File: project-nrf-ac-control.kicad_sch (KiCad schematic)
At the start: 8 parts, among them J1 SM04B-SRSS-TB(LF)(SN), Q1 SI2312BDS-T1-E3, U1 Pink Panda

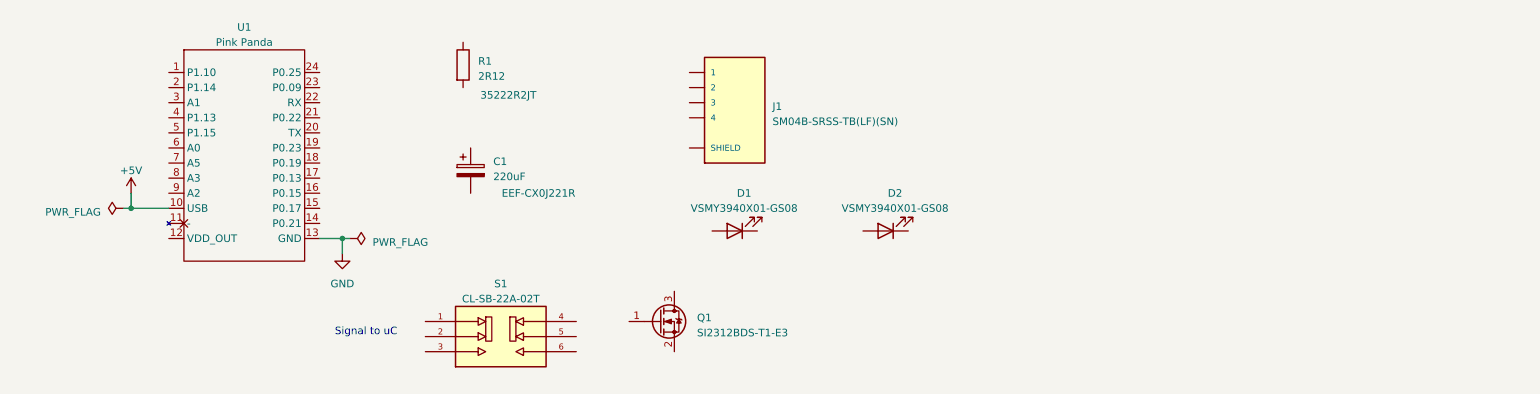
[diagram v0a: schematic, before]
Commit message: First draft schematic
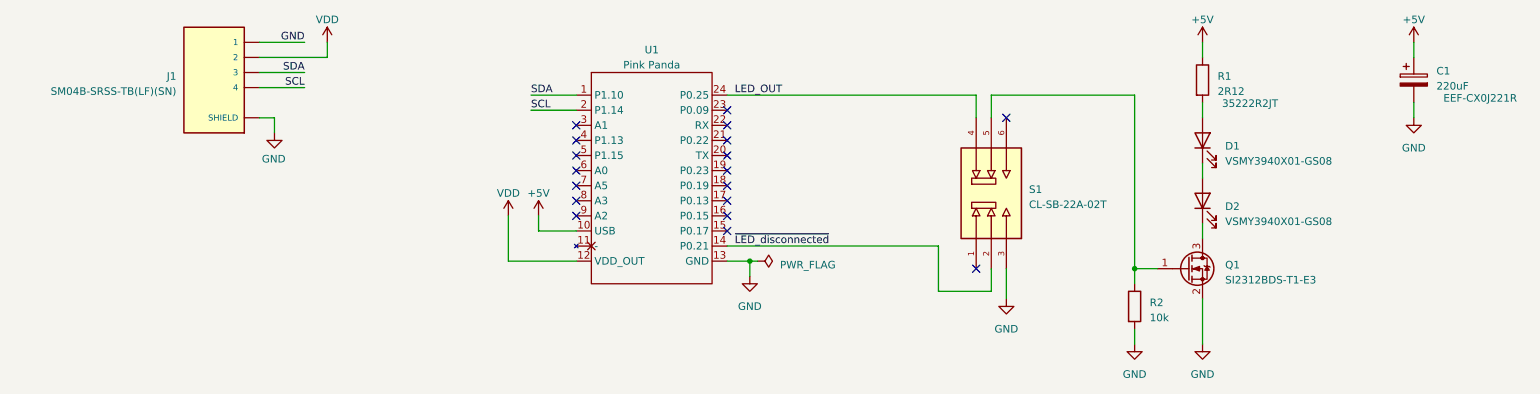
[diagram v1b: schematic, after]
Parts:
- added R2: 10k, symbol Device:R
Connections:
- net +5V: now also C1.1, R1.1
- net GND: now also C1.2, J1.1, J1.S1 (SHIELD), J1.S2 (SHIELD), Q1.2 (S), S1.3, R2.2
- net ~{LED_disconnected}: now reaches S1.2
- net ~{LED_disconnected}: now also U1.14 (P0.21)
- net LED_OUT: now reaches S1.4
- net LED_OUT: now also U1.24 (P0.25)
- net at S1.5: now also Q1.1 (G), R2.1
- net at R1.2: now also D1.2 (A)
- net SDA: now reaches U1.1 (P1.10)
- net SDA: now also J1.3
- net VDD: now reaches U1.12 (VDD_OUT)
- net VDD: now also J1.2
- net SCL: now reaches U1.2 (P1.14)
- net SCL: now also J1.4
- net at D1.1 (K): now also D2.2 (A)
- net at Q1.3 (D): now also D2.1 (K)
- no-connect marks 0 -> 18
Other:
- note removed: "Signal to uC"
- moved on the sheet: C1, D1, D2, J1, Q1, R1, S1, U1
